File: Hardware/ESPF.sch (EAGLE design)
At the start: 25 parts, among them IC1 CP2102N-A01-GQFN24, J1 USB-C-16P-16P, J2 ESPFLASH-1X6-2.54-PINS-RA, Q1 MMDT3904

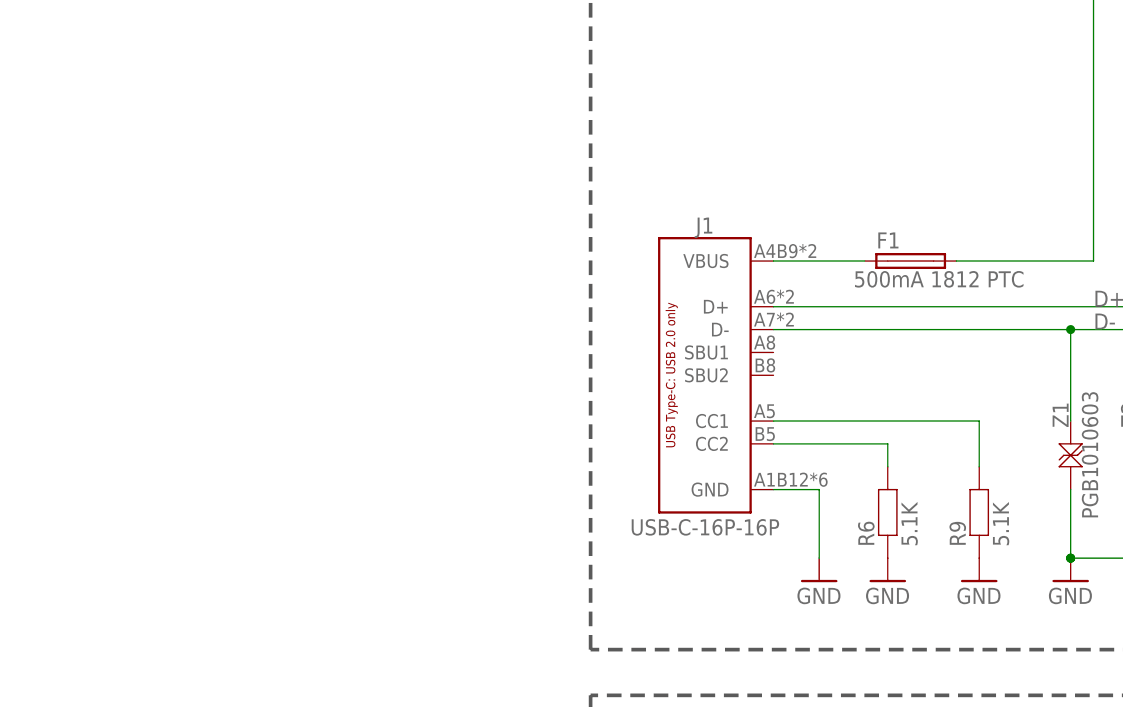
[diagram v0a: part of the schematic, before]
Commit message: Wurth_Connectors_WR-USB
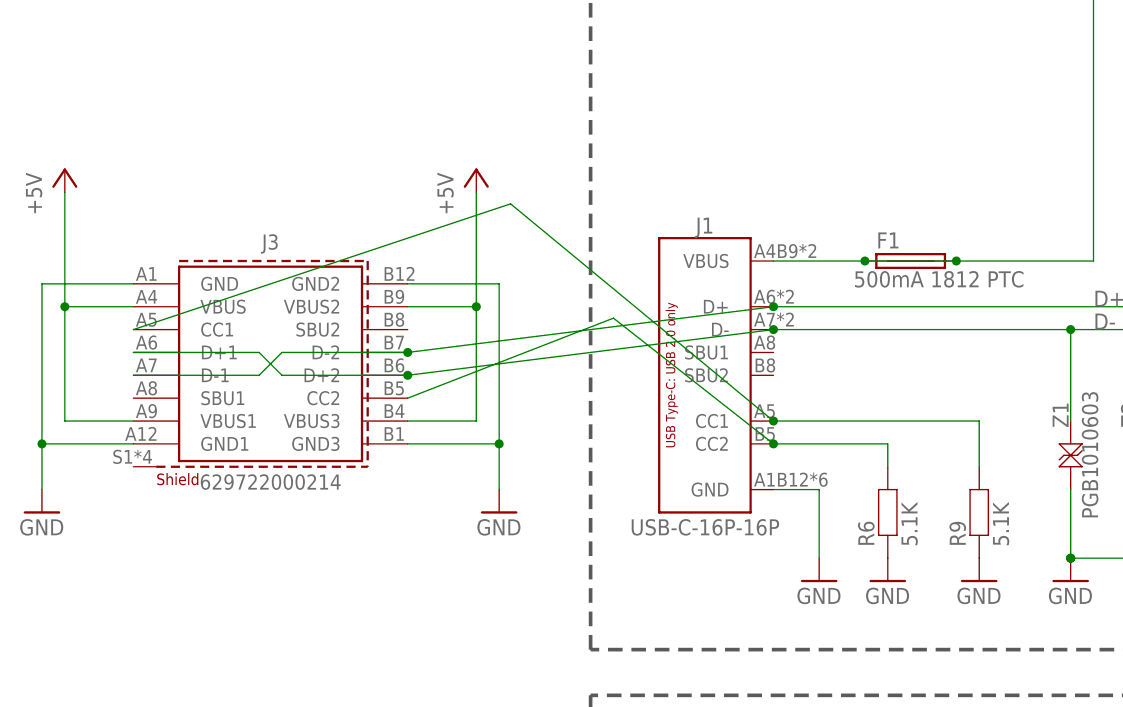
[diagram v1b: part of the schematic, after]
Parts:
- added J3: 629722000214, Wurth_Connectors_WR-USB:629722000214
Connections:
- removed net VIN: F1.1, J1.VBUS
- new net +5V: J3.VBUS, J3.VBUS1, J3.VBUS2, J3.VBUS3
- net 5V: now also F1.1, J1.VBUS
- net D+: now also J3.D-1, J3.D-2
- net D-: now also J3.D+1, J3.D+2
- net GND: now also J3.GND, J3.GND1, J3.GND2, J3.GND3
- net N$10: now also J3.CC1
- net N$9: now also J3.CC2
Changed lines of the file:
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@@
 <setting verticaltext="up"/>
 </settings>
-<grid distance="0.1" unitdist="inch" unit="inch" style="lines" multiple="1" display="no" altdistance="0.01" altunitdist="inch" altunit="inch"/>
+<grid distance="0.05" unitdist="inch" unit="inch" style="lines" multiple="1" display="yes" altdistance="0.01" altunitdist="inch" altunit="inch"/>
 <layers>
 <layer number="1" name="Top" color="4" fill="1" visible="no" active="no"/>
@@
 <part name="C3" library="SuperHouse-DiscreteSemi" library_urn="urn:adsk.eagle:library:11768461" deviceset="CAP" device="0603" package3d_urn="urn:adsk.eagle:package:7066315/6" value="100nF"/>
 <part name="GND10" library="SuperHouse-SupplySymbols" library_urn="urn:adsk.eagle:library:11790503" deviceset="GND" device=""/>
+<part name="J3" library="Wurth_Connectors_WR-USB" library_urn="urn:adsk.eagle:library:16513831" deviceset="629722000214" device="" package3d_urn="urn:adsk.eagle:package:32827710/4" value="629722000214"/>
+<part name="GND11" library="supply1" library_urn="urn:adsk.eagle:library:371" deviceset="GND" device=""/>
+<part name="GND12" library="supply1" library_urn="urn:adsk.eagle:library:371" deviceset="GND" device=""/>
+<part name="P+5" library="supply1" library_urn="urn:adsk.eagle:library:371" deviceset="+5V" device=""/>
+<part name="P+6" library="supply1" library_urn="urn:adsk.eagle:library:371" deviceset="+5V" device=""/>
 </parts>
 <sheets>
@@
 <attribute name="VALUE" x="193.04" y="91.44" size="1.778" layer="96"/>
 </instance>
+<instance part="J3" gate="G$1" x="-27.94" y="111.76" smashed="yes">
+<attribute name="NAME" x="-27.94" y="123.19" size="1.6764" layer="95" align="bottom-center"/>
+<attribute name="VALUE" x="-27.94" y="96.52" size="1.6764" layer="96" align="bottom-center"/>
+</instance>
+<instance part="GND11" gate="1" x="-53.34" y="93.98" smashed="yes">
+<attribute name="VALUE" x="-55.88" y="91.44" size="1.778" layer="96"/>
+</instance>
+<instance part="GND12" gate="1" x="-2.54" y="93.98" smashed="yes">
+<attribute name="VALUE" x="-5.08" y="91.44" size="1.778" layer="96"/>
+</instance>
+<instance part="P+5" gate="1" x="-50.8" y="132.08" smashed="yes">
+<attribute name="VALUE" x="-53.34" y="127" size="1.778" layer="96" rot="R90"/>
+</instance>
+<instance part="P+6" gate="1" x="-5.08" y="132.08" smashed="yes">
+<attribute name="VALUE" x="-7.62" y="127" size="1.778" layer="96" rot="R90"/>
+</instance>
 </instances>
 <busses>
@@
 <pinref part="F1" gate="A" pin="2"/>
 <wire x1="63.5" y1="121.92" x2="48.26" y2="121.92" width="0.1524" layer="91"/>
+<pinref part="F1" gate="A" pin="1"/>
+<pinref part="J1" gate="G$1" pin="VBUS"/>
+<wire x1="27.94" y1="121.92" x2="38.1" y2="121.92" width="0.1524" layer="91"/>
+<wire x1="38.1" y1="121.92" x2="48.26" y2="121.92" width="0.1524" layer="91"/>
+<junction x="38.1" y="121.92"/>
+<junction x="48.26" y="121.92"/>
 </segment>
 <segment>
@@
 <wire x1="195.58" y1="96.52" x2="195.58" y2="104.14" width="0.1524" layer="91"/>
 </segment>
+<segment>
+<pinref part="J3" gate="G$1" pin="GND"/>
+<wire x1="-43.18" y1="119.38" x2="-53.34" y2="119.38" width="0.1524" layer="91"/>
+<wire x1="-53.34" y1="119.38" x2="-53.34" y2="101.6" width="0.1524" layer="91"/>
+<pinref part="GND11" gate="1" pin="GND"/>
+<pinref part="J3" gate="G$1" pin="GND1"/>
+<wire x1="-53.34" y1="101.6" x2="-53.34" y2="96.52" width="0.1524" layer="91"/>
+<wire x1="-43.18" y1="101.6" x2="-53.34" y2="101.6" width="0.1524" layer="91"/>
+<junction x="-53.34" y="101.6"/>
+</segment>
+<segment>
+<pinref part="J3" gate="G$1" pin="GND2"/>
+<wire x1="-12.7" y1="119.38" x2="-2.54" y2="119.38" width="0.1524" layer="91"/>
+<wire x1="-2.54" y1="119.38" x2="-2.54" y2="101.6" width="0.1524" layer="91"/>
+<pinref part="GND12" gate="1" pin="GND"/>
+<pinref part="J3" gate="G$1" pin="GND3"/>
+<wire x1="-2.54" y1="101.6" x2="-2.54" y2="96.52" width="0.1524" layer="91"/>
+<wire x1="-12.7" y1="101.6" x2="-2.54" y2="101.6" width="0.1524" layer="91"/>
+<junction x="-2.54" y="101.6"/>
+</segment>
 </net>
 <net name="D-" class="0">
@@
 <pinref part="J1" gate="G$1" pin="D-"/>
 <wire x1="27.94" y1="114.3" x2="60.96" y2="114.3" width="0.1524" layer="91"/>
+<pinref part="J3" gate="G$1" pin="D+2"/>
+<wire x1="-12.7" y1="109.22" x2="-26.67" y2="109.22" width="0.1524" layer="91"/>
+<wire x1="-26.67" y1="109.22" x2="-29.21" y2="111.76" width="0.1524" layer="91"/>
+<pinref part="J3" gate="G$1" pin="D+1"/>
+<wire x1="-29.21" y1="111.76" x2="-43.18" y2="111.76" width="0.1524" layer="91"/>
+<wire x1="27.94" y1="114.3" x2="-12.7" y2="109.22" width="0.1524" layer="91"/>
+<junction x="27.94" y="114.3"/>
+<junction x="-12.7" y="109.22"/>
 </segment>
 </net>
@@
 <pinref part="J1" gate="G$1" pin="D+"/>
 <wire x1="68.58" y1="116.84" x2="27.94" y2="116.84" width="0.1524" layer="91"/>
+<pinref part="J3" gate="G$1" pin="D-1"/>
+<wire x1="-43.18" y1="109.22" x2="-29.21" y2="109.22" width="0.1524" layer="91"/>
+<pinref part="J3" gate="G$1" pin="D-2"/>
+<wire x1="-12.7" y1="111.76" x2="-26.67" y2="111.76" width="0.1524" layer="91"/>
+<wire x1="-26.67" y1="111.76" x2="-29.21" y2="109.22" width="0.1524" layer="91"/>
+<wire x1="-12.7" y1="111.76" x2="27.94" y2="116.84" width="0.1524" layer="91"/>
+<junction x="-12.7" y="111.76"/>
+<junction x="27.94" y="116.84"/>
 </segment>
 </net>
@@
 </segment>
 </net>
-<net name="VIN" class="0">
-<segment>
-<pinref part="F1" gate="A" pin="1"/>
-<pinref part="J1" gate="G$1" pin="VBUS"/>
-<wire x1="27.94" y1="121.92" x2="38.1" y2="121.92" width="0.1524" layer="91"/>
-</segment>
-</net>
 <net name="N$6" class="0">
 <segment>
@@
 <wire x1="27.94" y1="101.6" x2="40.64" y2="101.6" width="0.1524" layer="91"/>
 <wire x1="40.64" y1="101.6" x2="40.64" y2="99.06" width="0.1524" layer="91"/>
+<pinref part="J3" gate="G$1" pin="CC2"/>
+<wire x1="-12.7" y1="106.68" x2="10.16" y2="115.57" width="0.1524" layer="91"/>
+<wire x1="10.16" y1="115.57" x2="27.94" y2="101.6" width="0.1524" layer="91"/>
+<junction x="27.94" y="101.6"/>
 </segment>
 </net>
@@
 <wire x1="27.94" y1="104.14" x2="50.8" y2="104.14" width="0.1524" layer="91"/>
 <wire x1="50.8" y1="104.14" x2="50.8" y2="99.06" width="0.1524" layer="91"/>
-</segment>
-</net>
+<pinref part="J3" gate="G$1" pin="CC1"/>
+<wire x1="27.94" y1="104.14" x2="-1.27" y2="128.27" width="0.1524" layer="91"/>
+<wire x1="-1.27" y1="128.27" x2="-43.18" y2="114.3" width="0.1524" layer="91"/>
+<junction x="27.94" y="104.14"/>
+</segment>
+</net>
+<net name="+5V" class="0">
+<segment>
+<pinref part="J3" gate="G$1" pin="VBUS"/>
+<wire x1="-50.8" y1="116.84" x2="-43.18" y2="116.84" width="0.1524" layer="91"/>
+<pinref part="J3" gate="G$1" pin="VBUS1"/>
+<wire x1="-43.18" y1="104.14" x2="-50.8" y2="104.14" width="0.1524" layer="91"/>
+<wire x1="-50.8" y1="104.14" x2="-50.8" y2="116.84" width="0.1524" layer="91"/>
+<wire x1="-50.8" y1="116.84" x2="-50.8" y2="129.54" width="0.1524" layer="91"/>
+<junction x="-50.8" y="116.84"/>
+<pinref part="P+5" gate="1" pin="+5V"/>
+</segment>
+<segment>
+<pinref part="J3" gate="G$1" pin="VBUS3"/>
+<wire x1="-12.7" y1="104.14" x2="-5.08" y2="104.14" width="0.1524" layer="91"/>
+<wire x1="-5.08" y1="104.14" x2="-5.08" y2="116.84" width="0.1524" layer="91"/>
+<pinref part="J3" gate="G$1" pin="VBUS2"/>
+<wire x1="-5.08" y1="116.84" x2="-5.08" y2="129.54" width="0.1524" layer="91"/>
+<wire x1="-12.7" y1="116.84" x2="-5.08" y2="116.84" width="0.1524" layer="91"/>
+<junction x="-5.08" y="116.84"/>
+<pinref part="P+6" gate="1" pin="+5V"/>
+</segment>
+</net>
